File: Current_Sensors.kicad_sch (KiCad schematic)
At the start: 12 parts

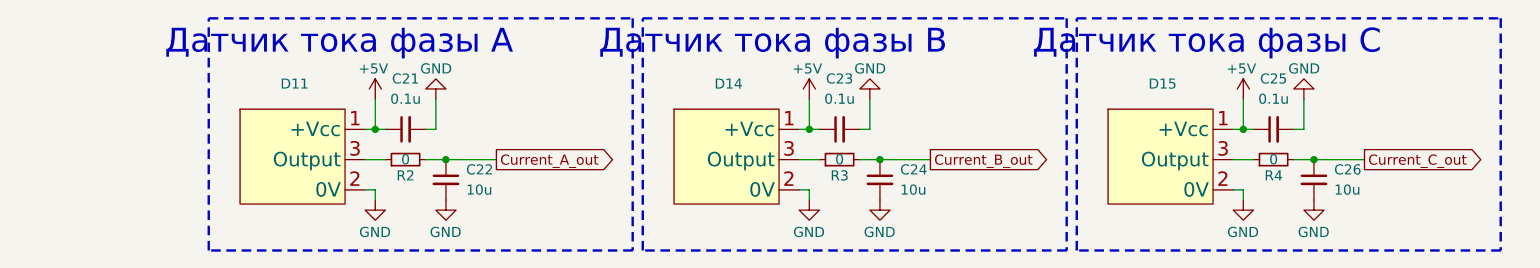
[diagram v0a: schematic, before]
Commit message: VER2.2.1: создал папку для производственных доков
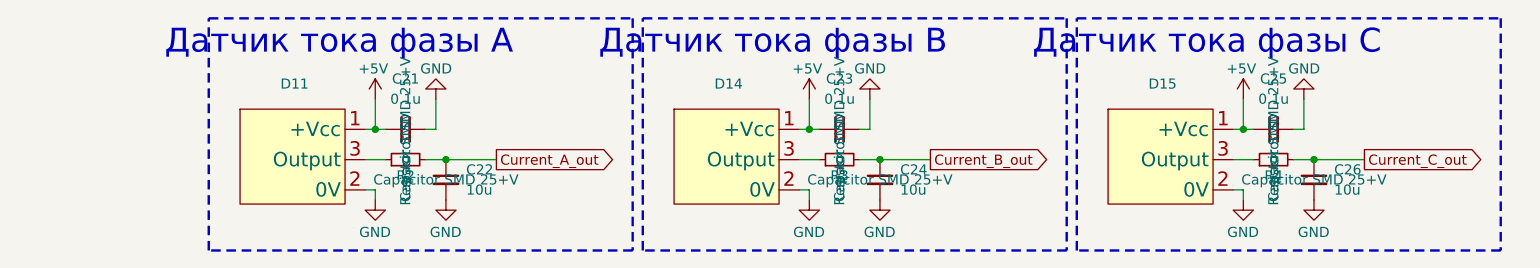
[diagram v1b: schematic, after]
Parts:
- C21, C22, C23, C24, C25, C26: Description P/N (none) -> Capacitor SMD 25+V
- R2, R3, R4: Description P/N (none) -> Resistor SMD
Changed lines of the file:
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@@
 			)
 		)
-		(property "Description P/N" ""
+		(property "Description P/N" "Capacitor SMD 25+V"
 			(at 156.21 111.76 0)
 			(effects
@@
 			)
 		)
-		(property "Description P/N" ""
+		(property "Description P/N" "Capacitor SMD 25+V"
 			(at 101.6 111.76 0)
 			(effects
@@
 			)
 		)
-		(property "Description P/N" ""
+		(property "Description P/N" "Capacitor SMD 25+V"
 			(at 151.13 105.41 0)
 			(effects
@@
 			)
 		)
-		(property "Description P/N" ""
+		(property "Description P/N" "Capacitor SMD 25+V"
 			(at 205.74 105.41 0)
 			(effects
@@
 			)
 		)
-		(property "Description P/N" ""
+		(property "Description P/N" "Resistor SMD"
 			(at 205.74 109.22 0)
 			(effects
@@
 			)
 		)
-		(property "Description P/N" ""
+		(property "Description P/N" "Capacitor SMD 25+V"
 			(at 210.82 111.76 0)
 			(effects
@@
 			)
 		)
-		(property "Description P/N" ""
+		(property "Description P/N" "Resistor SMD"
 			(at 151.13 109.22 0)
 			(effects
@@
 			)
 		)
-		(property "Description P/N" ""
+		(property "Description P/N" "Resistor SMD"
 			(at 96.52 109.22 0)
 			(effects
@@
 			)
 		)
-		(property "Description P/N" ""
+		(property "Description P/N" "Capacitor SMD 25+V"
 			(at 96.52 105.41 0)
 			(effects

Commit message: VER2.2.1: исправил все доки
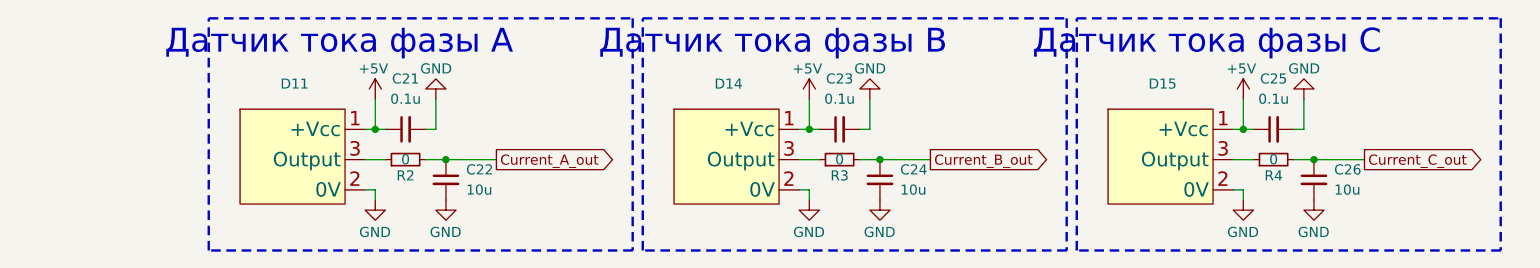
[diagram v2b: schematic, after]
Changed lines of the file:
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@@
 		(date "2025-06-04")
 		(company "ООО \"ЭТТ\"")
+		(comment 1 "НВЦТ.EVP150-2-1.2000.120_v1 Э3")
 	)
 	(rectangle
@@
 					(size 1.27 1.27)
 				)
+				(hide yes)
 			)
 		)
@@
 					(size 1.27 1.27)
 				)
+				(hide yes)
 			)
 		)
@@
 					(size 1.27 1.27)
 				)
+				(hide yes)
 			)
 		)
@@
 					(size 1.27 1.27)
 				)
+				(hide yes)
 			)
 		)
@@
 					(size 1.27 1.27)
 				)
+				(hide yes)
 			)
 		)
@@
 					(size 1.27 1.27)
 				)
+				(hide yes)
 			)
 		)
@@
 					(size 1.27 1.27)
 				)
+				(hide yes)
 			)
 		)
@@
 					(size 1.27 1.27)
 				)
+				(hide yes)
 			)
 		)
@@
 					(size 1.27 1.27)
 				)
-			)
-		)
+				(hide yes)
+			)
+		)
